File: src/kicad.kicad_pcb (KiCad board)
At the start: 2 copper layers, 90.4 x 126.5 mm, 6 parts

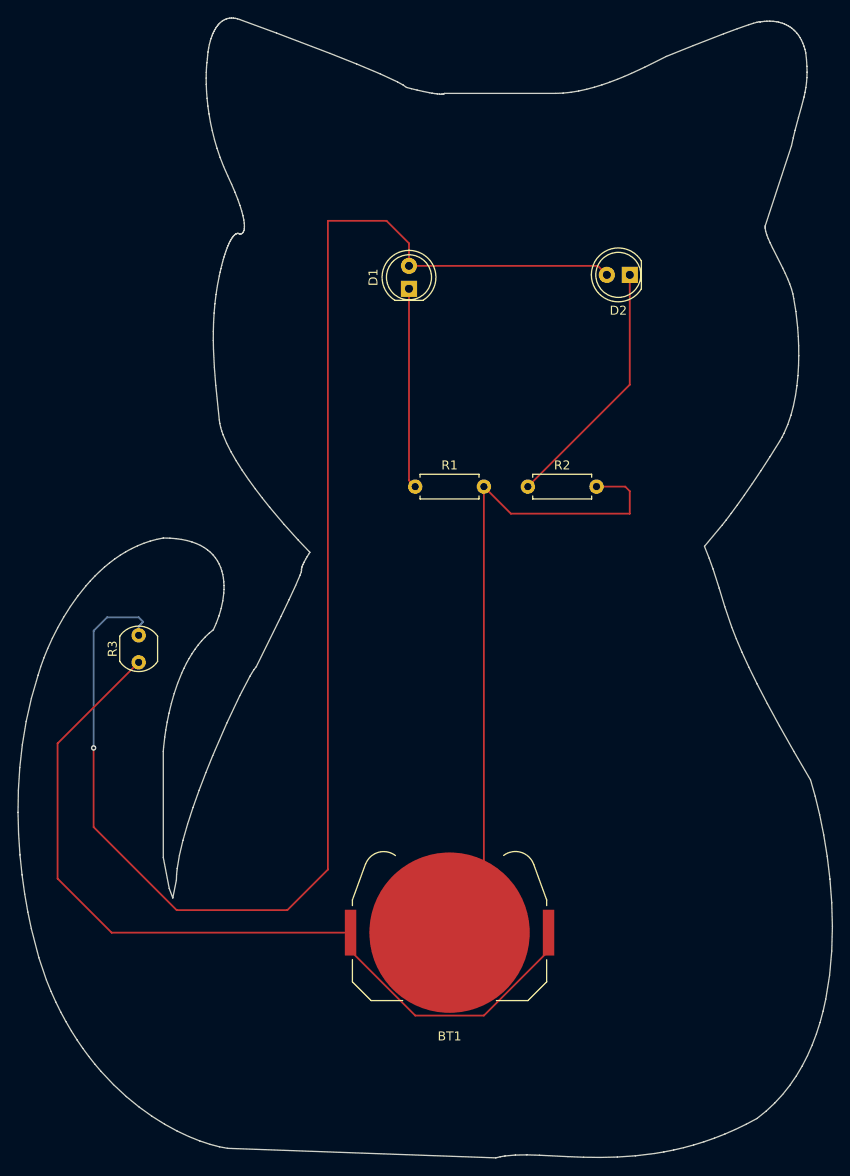
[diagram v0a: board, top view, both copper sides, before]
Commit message: update PCB
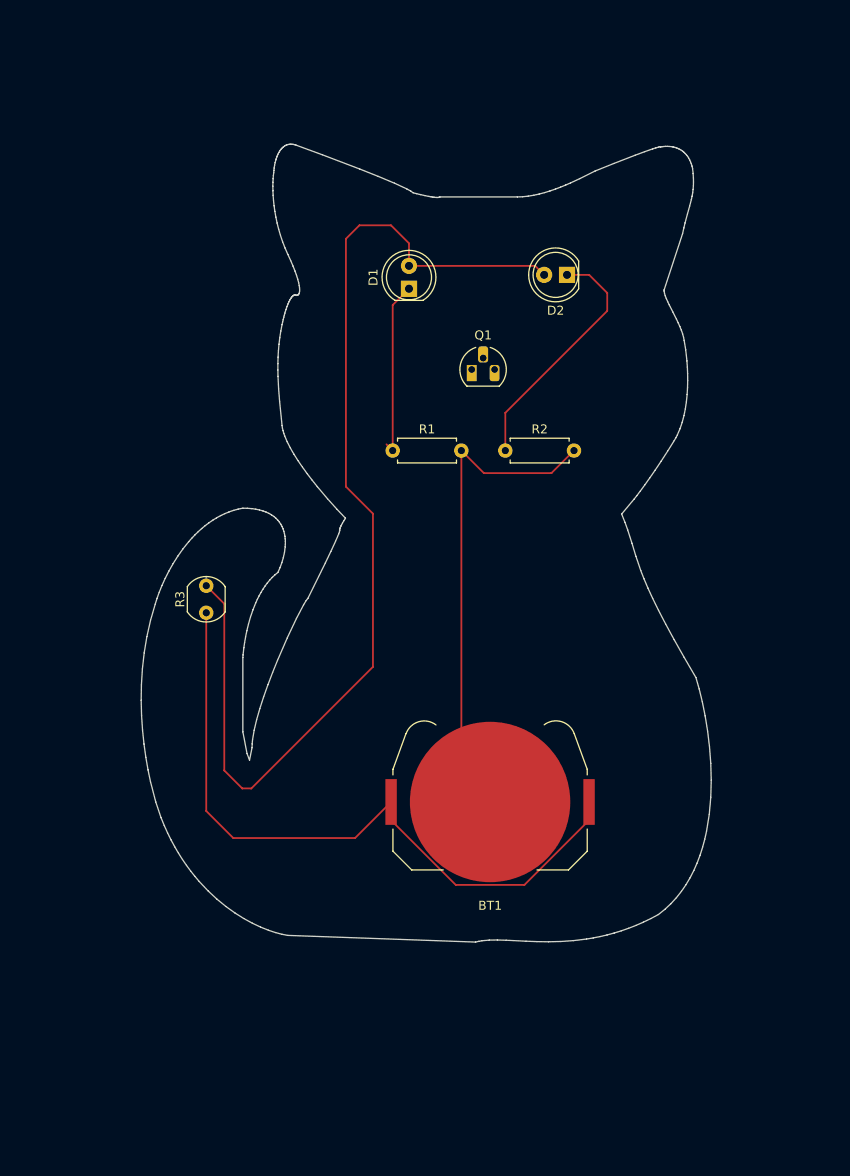
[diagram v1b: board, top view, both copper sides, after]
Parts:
- added Q1: NPN, Package_TO_SOT_THT:TO-92L_HandSolder, F.Cu at (76.0, 89.0)
- moved BT1 15.2 mm to (78.0, 137.0)
- moved R3 9.30 mm to (46.5, 116.0)
- moved D2 6.96 mm to (86.5, 78.5)
- moved R1 4.72 mm to (67.2, 98.0)
- moved R2 4.72 mm to (79.7, 98.0)
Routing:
- net Net-(D1-A): track 168.4 -> 120.4 mm, vias 1 -> 0
- net Net-(BT1--): track 74.9 -> 54.9 mm
- net Net-(BT1-+): track 94.7 -> 77.4 mm
- net Net-(D1-K): track 22.2 -> 19.7 mm
- net Net-(D2-K): track 28.2 -> 27.5 mm
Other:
- board size 90.4 x 126.5 mm -> 63.3 x 88.6 mm
